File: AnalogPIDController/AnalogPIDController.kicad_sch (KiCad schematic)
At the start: 32 parts, among them Q1 Q_NPN, U1 TL082, U2 TL084

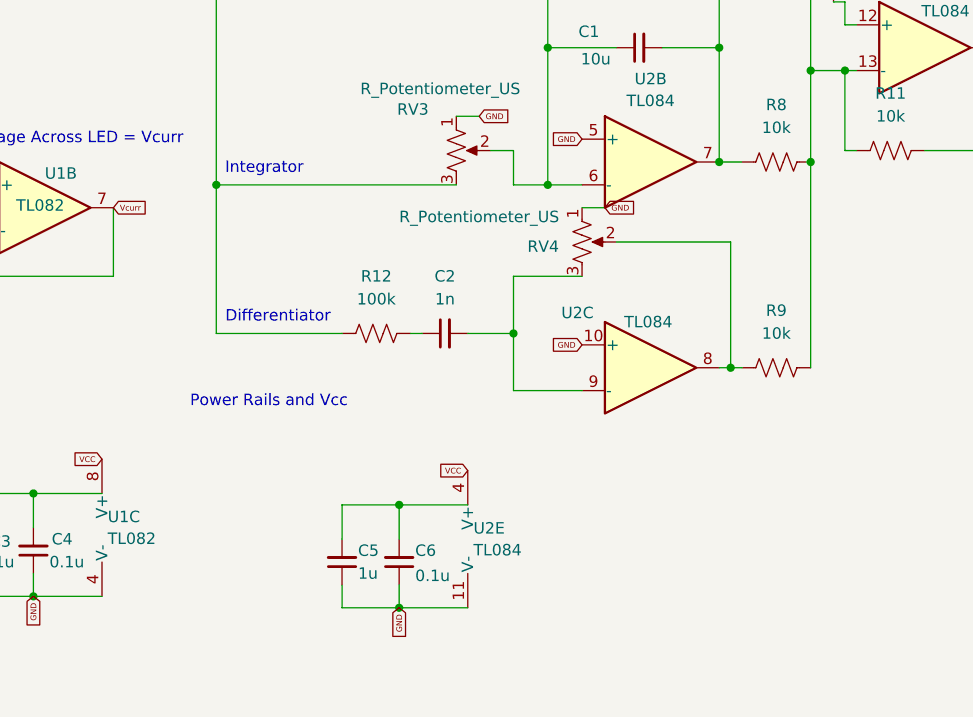
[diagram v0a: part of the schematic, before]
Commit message: fixes
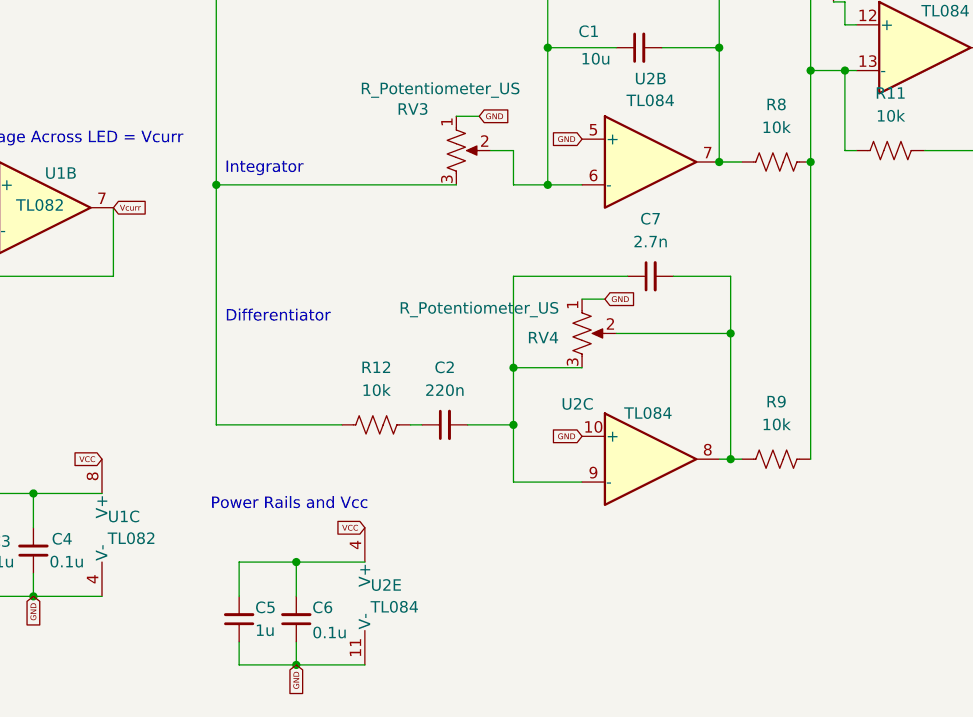
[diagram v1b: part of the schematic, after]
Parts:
- added C7: 2.7n, symbol Device:C_Small
- C2: value 1n -> 220n
- R12: value 100k -> 10k
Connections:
- net at R9.1, RV4.2, U2.8: now also C7.2
- net at C2.2, RV4.3, U2.9 (-): now also C7.1
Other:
- moved on the sheet: C2, C5, C6, R12, R9, RV4, U2C, U2E
